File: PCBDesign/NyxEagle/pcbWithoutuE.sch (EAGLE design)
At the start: 35 parts, among them IC1 DRV8304SRHAR

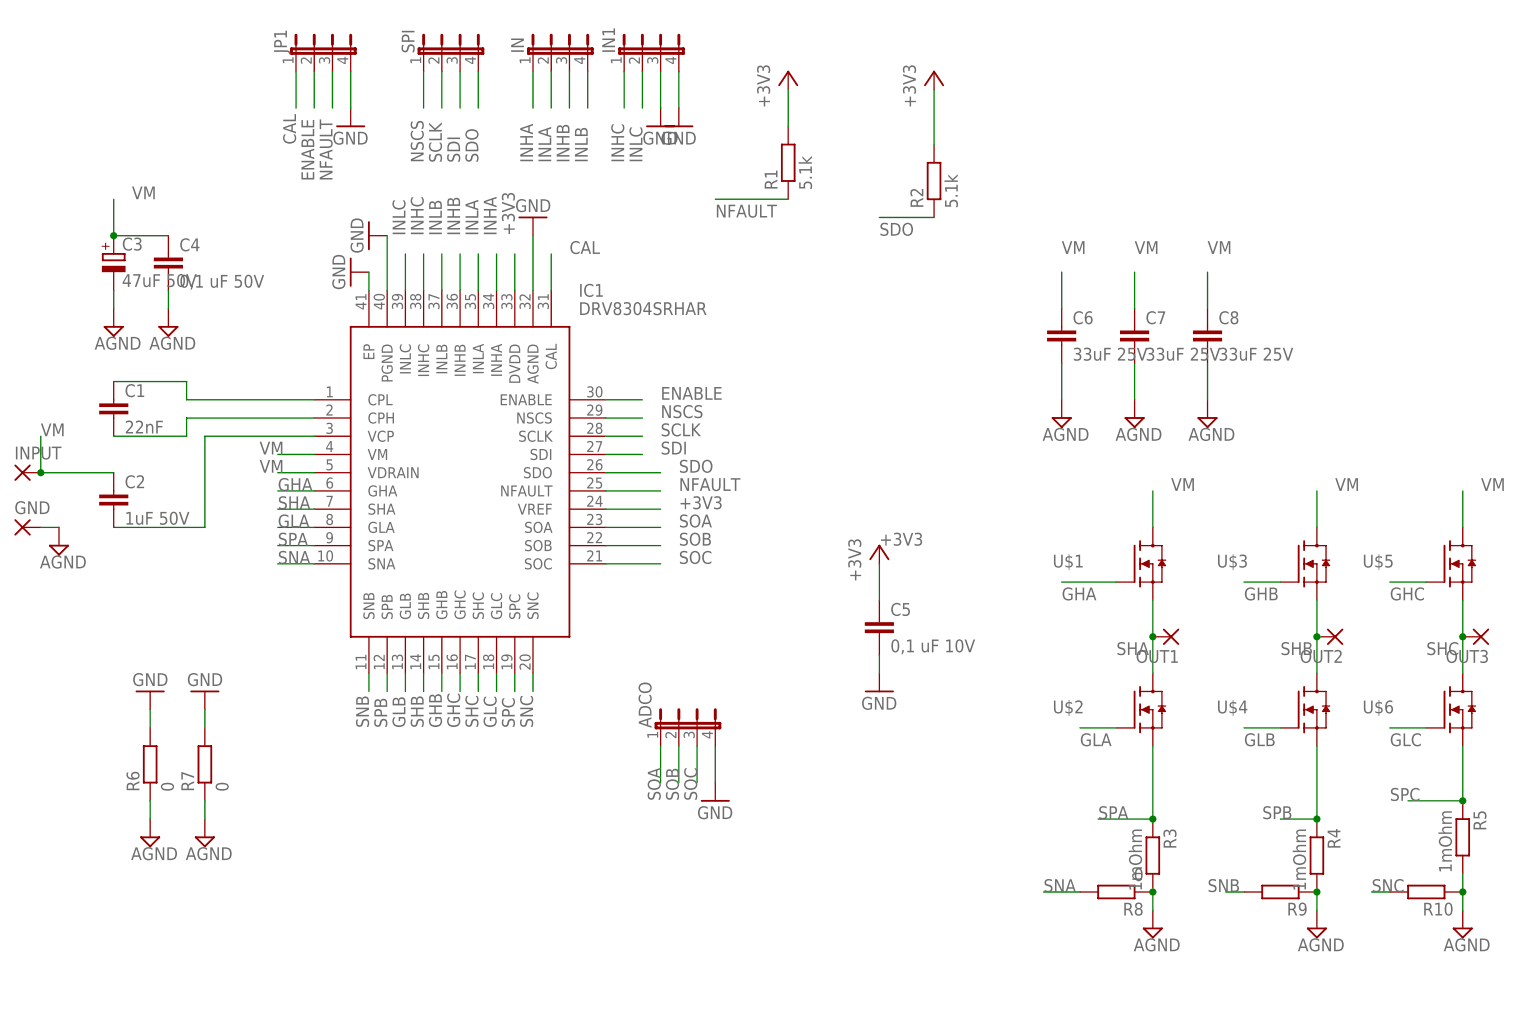
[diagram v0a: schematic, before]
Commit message: Update mul_s32_hiSR.h, queue.c, and 59 more files...
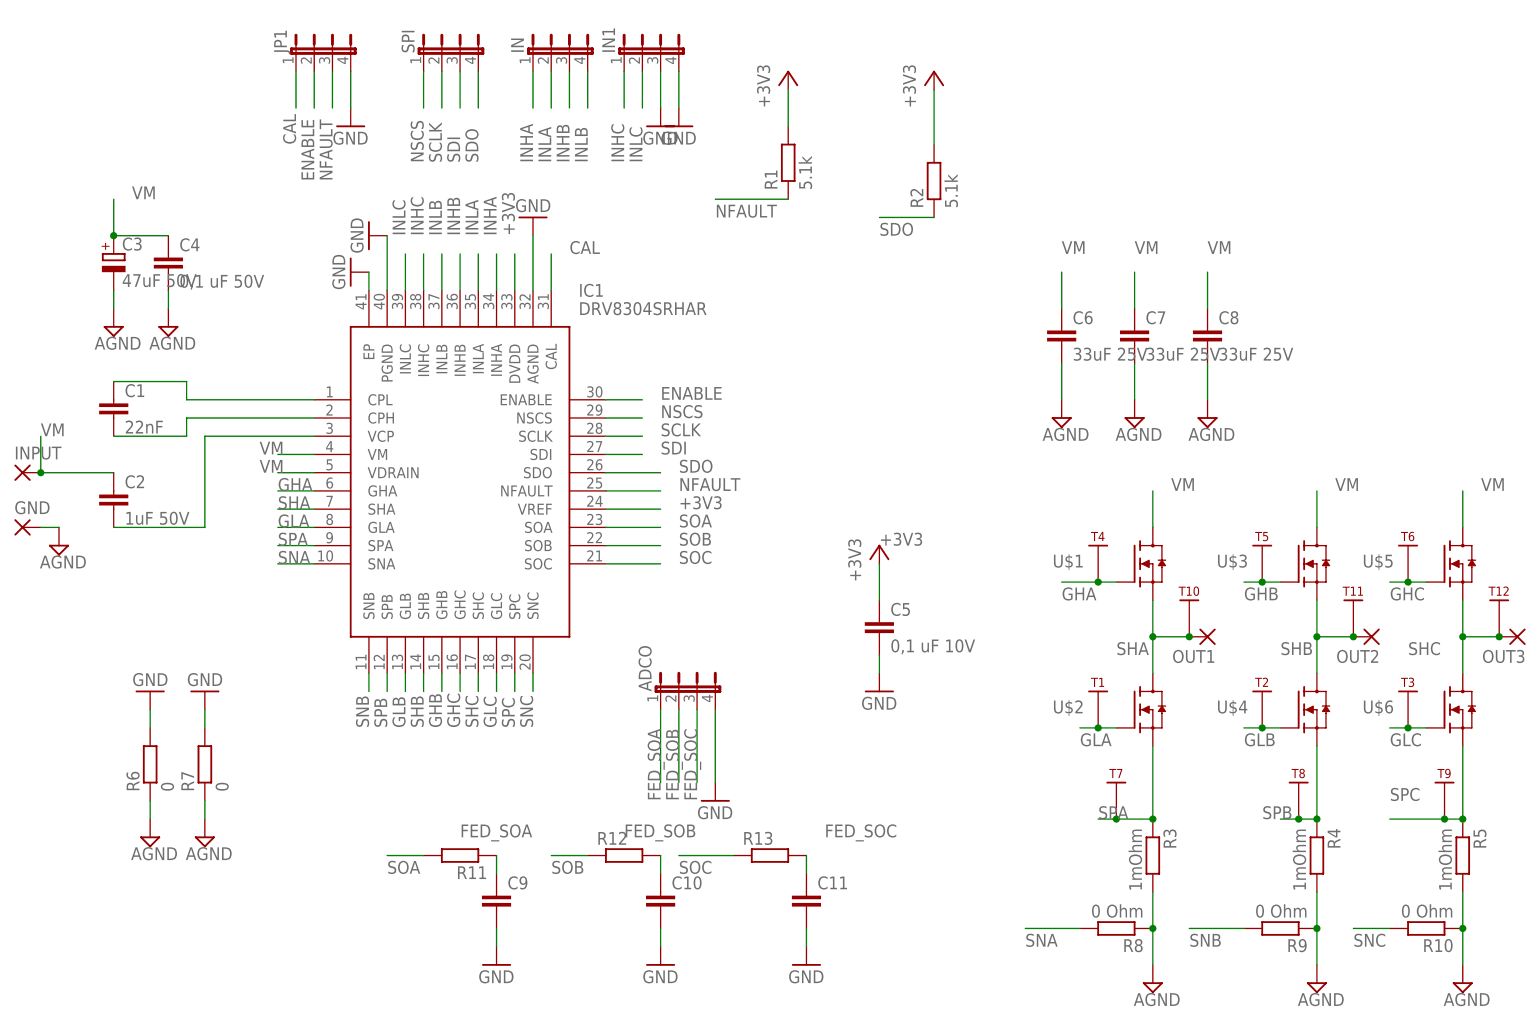
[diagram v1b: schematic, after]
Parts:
- added C10, C11, C9: (no value), resistor:C-EUC0805
- added R11, R12, R13: (no value), resistor:R-EU_R0805
- added T1, T10, T11, T12, T2, T3, T4, T5, T6, T7, T8, T9: TEST_POINT1593, ERIC:TEST_POINT1593
- R10, R9: value (none) -> 0 Ohm; device rcl:R-EU_R0201 -> resistor:R-EU_R0603
- R8: value 0 -> 0 Ohm; device rcl:R-EU_R0201 -> resistor:R-EU_R0603
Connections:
- new net FED_SOA: ADCO.1, C9.1, R11.1
- new net FED_SOB: ADCO.2, C10.1, R12.2
- new net FED_SOC: ADCO.3, C11.1, R13.2
- net GHA: now also T4.1
- net GHB: now also T5.1
- net GHC: now also T6.1
- net GLA: now also T1.1
- net GLB: now also T2.1
- net GLC: now also T3.1
- net GND: now also C10.2, C11.2, C9.2
- net SHA: now also T10.1
- net SHB: now also T11.1
- net SHC: now also T12.1
- net SOA: now also R11.2; no longer ADCO.1
- net SOB: now also R12.1; no longer ADCO.2
- net SOC: now also R13.1; no longer ADCO.3
- net SPA: now also T7.1
- net SPB: now also T8.1
- net SPC: now also T9.1
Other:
- moved on the sheet: ADCO, OUT1, OUT2, OUT3, R10, R5, R8, R9
